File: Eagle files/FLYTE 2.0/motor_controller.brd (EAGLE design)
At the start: 66 x 56 mm, 21 parts, among them J1 XT60PW-F

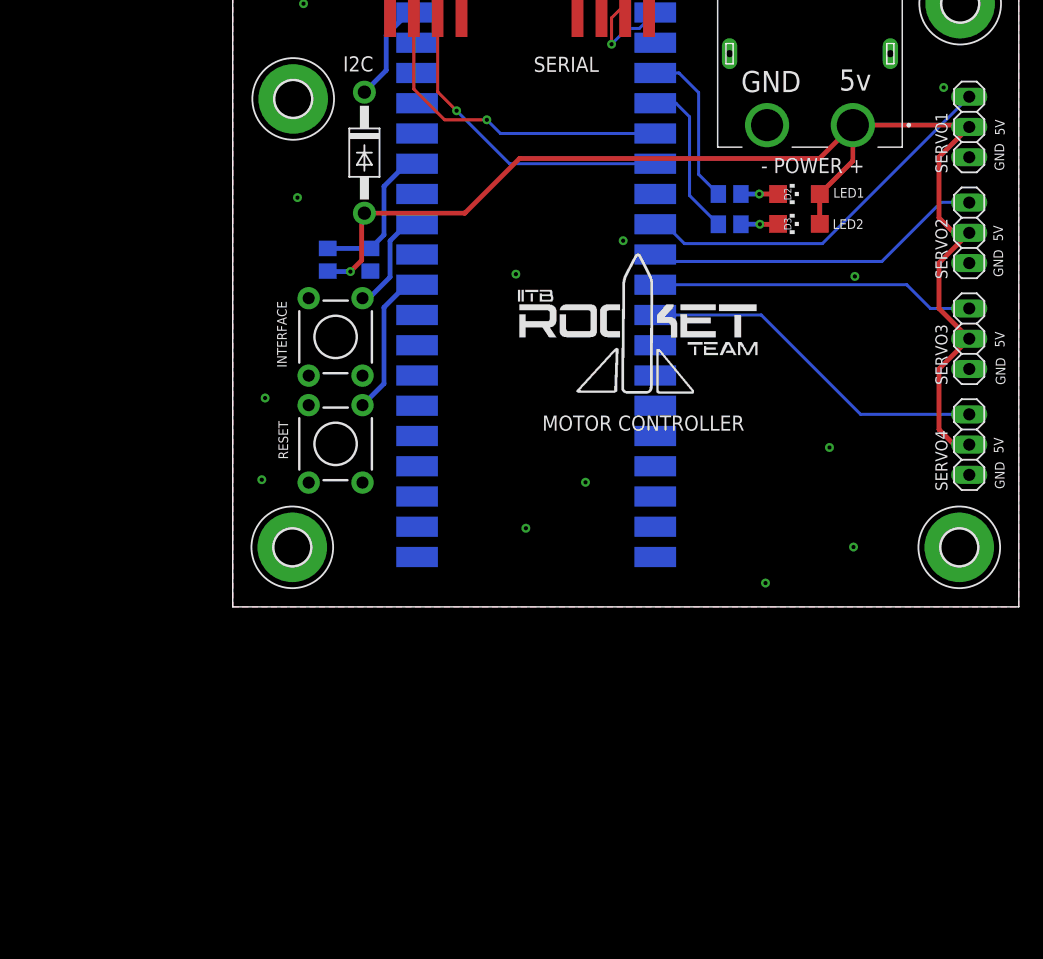
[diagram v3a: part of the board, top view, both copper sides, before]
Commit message: idk
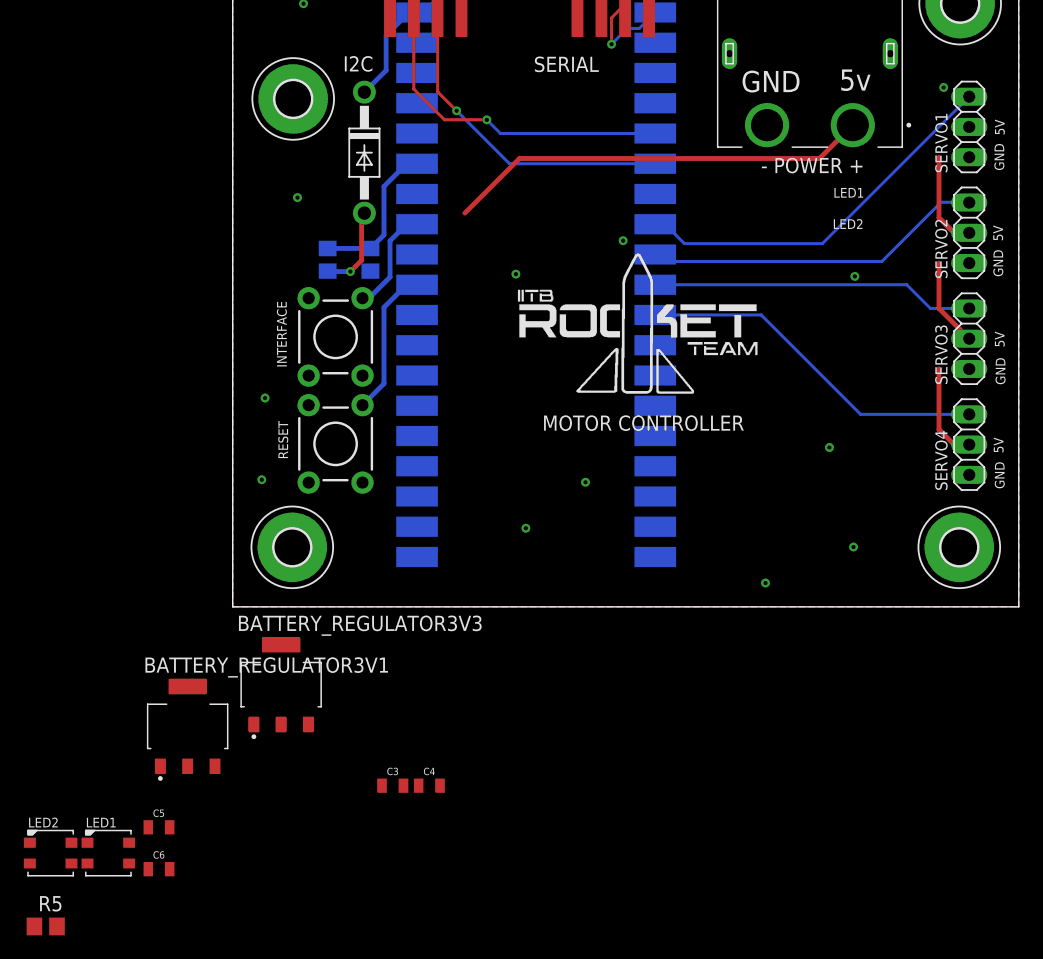
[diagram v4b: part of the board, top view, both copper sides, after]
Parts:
- removed D2, D3: (no value), led:CHIPLED_1206
- removed R3, R4: (no value), rcl:R0805
- added BATTERY_REGULATOR3V1, BATTERY_REGULATOR3V3: AMS1117-3.3, AMS1117-3.3:SOT229P700X180-4N
- added C3, C4, C5, C6: 22uF, SparkFun-Capacitors:0805
- added LED1, LED2: WS2812B3535, WS2812B:LED3535
- added R5: 4.7v, rcl:R0805
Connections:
- removed net LED1: PICO.P$4, R3.1
- removed net LED2: PICO.P$5, R4.1
- removed net N$5: D2.C, R3.2
- removed net N$6: D3.C, R4.2
- new net 3.3V: R2.1
- new net 3V3: BATTERY_REGULATOR3V3.2, C3.2, D1.A
- new net 7.4V: BATTERY_REGULATOR3V1.3, BATTERY_REGULATOR3V3.3, C4.2, C5.2, J1.1, SERVO1.2, SERVO2.2, SERVO3.2, SERVO4.2
- new net LED: PICO.P$20, R5.2
- new net N$7: LED1.3, LED2.1
- new net N$8: LED1.1, R5.1
- net 5V: now also BATTERY_REGULATOR3V1.2, C6.2, LED1.2, LED2.2; no longer D1.A, D2.A, D3.A, J1.1, R2.1, SERVO1.2, SERVO2.2, SERVO3.2, SERVO4.2
- net GND: now also BATTERY_REGULATOR3V1.1, BATTERY_REGULATOR3V3.1, C3.1, C4.1, C5.1, C6.1, LED1.4, LED2.4
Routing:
- net 5V: track 105.1 -> 0.00 mm, vias 1 -> 0
- net 7.4V: track 0.00 -> 59.6 mm
- net LED1: track 13.5 -> 0.00 mm
- net LED2: track 13.4 -> 0.00 mm
- net 3.3V: track 0.00 -> 6.99 mm, vias 0 -> 1
- net N$6: track 3.13 -> 0.00 mm, vias 1 -> 0
- net N$5: track 3.12 -> 0.00 mm, vias 1 -> 0
